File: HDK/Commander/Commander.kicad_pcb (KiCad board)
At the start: 2 copper layers, 45 x 20 mm, 47 parts, among them J1 SWD, J3 FPC0.5-SMT-8, SW1 NRST, SW2 BOOT0, U1 STM32G431CBU6, U3 W25Q128JVS, Y1 8M, Y2 32.768K

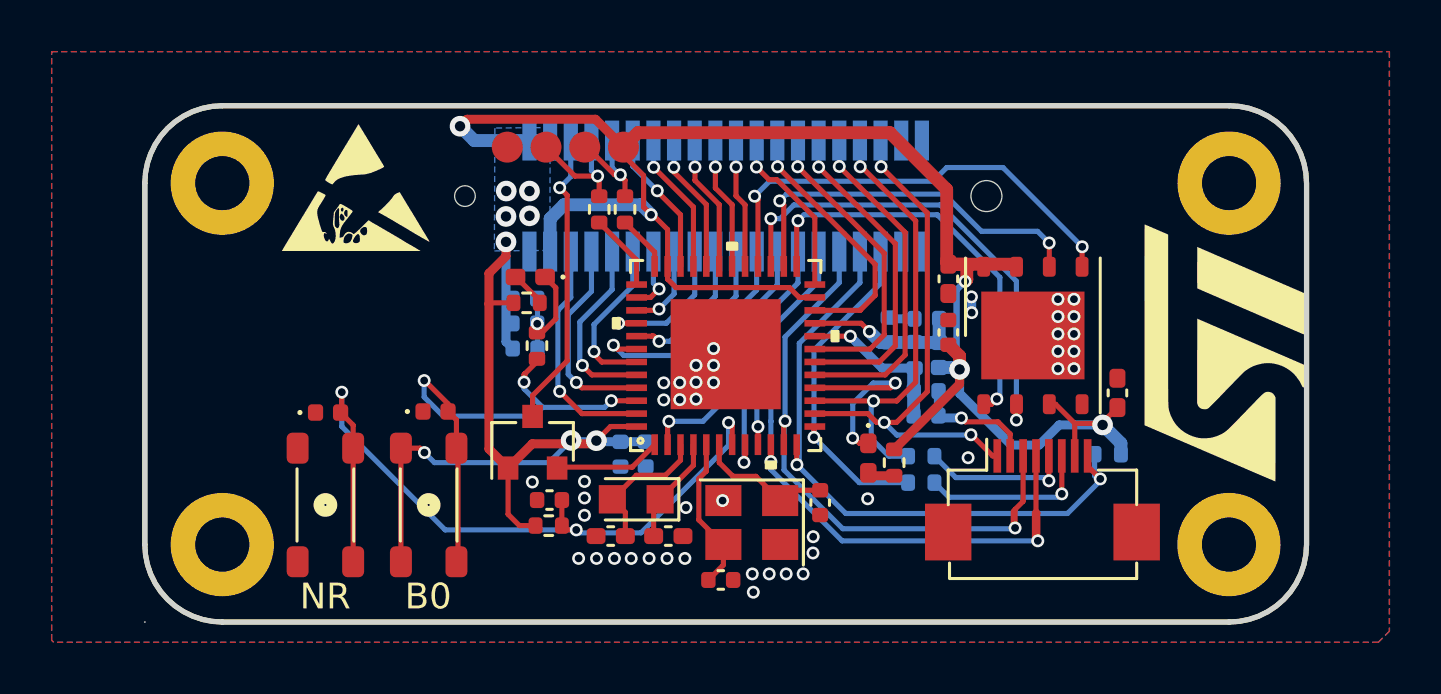
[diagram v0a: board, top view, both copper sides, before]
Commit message: Update Commander
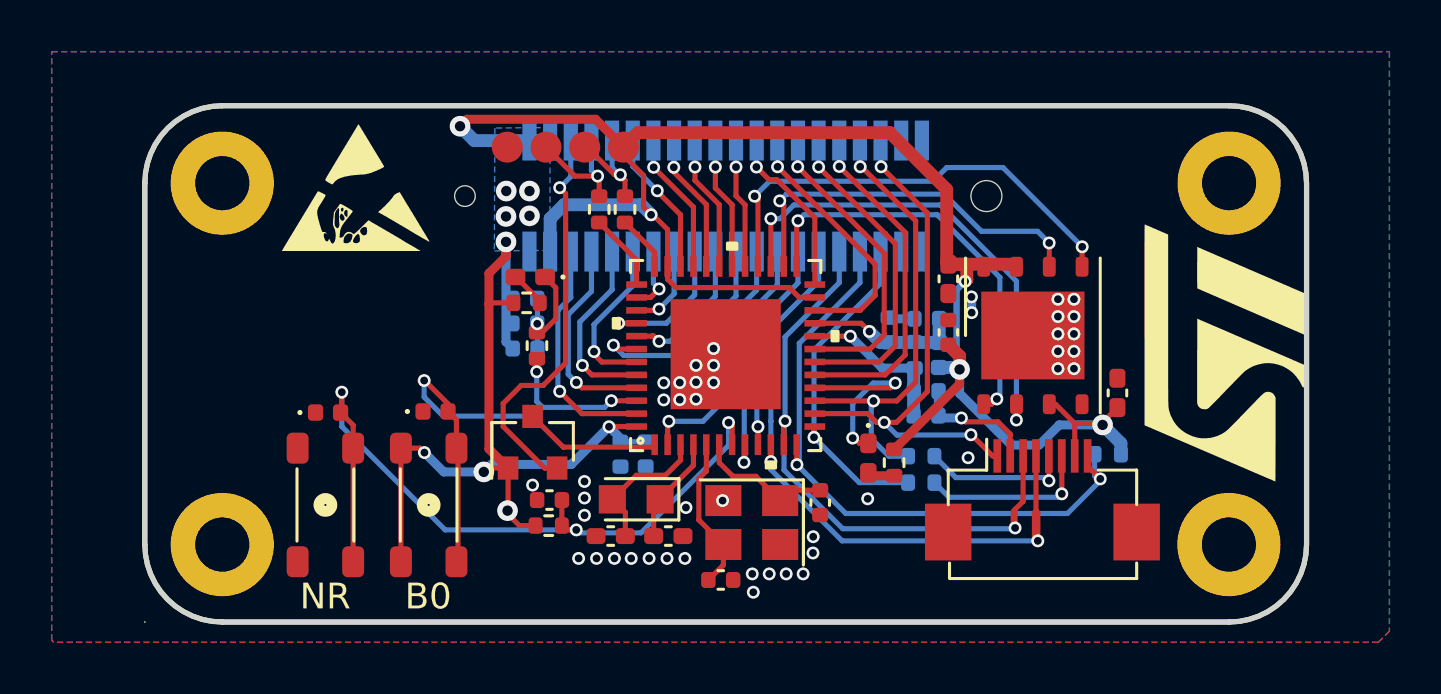
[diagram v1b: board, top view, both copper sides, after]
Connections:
- D1 pad 2: /VBAT+ -> /VBAT_Pin
- D1 pad 3: /VBAT_Pin -> /VBAT+
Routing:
- net /VBAT_Pin: track 11.5 -> 15.6 mm
- net +3V3: track 109.9 -> 106.9 mm, vias 13 -> 14
- net /VBAT+: track 4.11 -> 5.26 mm
- net /BOOT0: track 19.6 -> 19.0 mm
